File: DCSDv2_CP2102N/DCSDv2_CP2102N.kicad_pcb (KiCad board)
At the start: 2 copper layers, 37 x 27 mm, 18 parts, among them P1 USB_C_Plug_USB2.0, U1 CP2102N-Axx-xQFN28

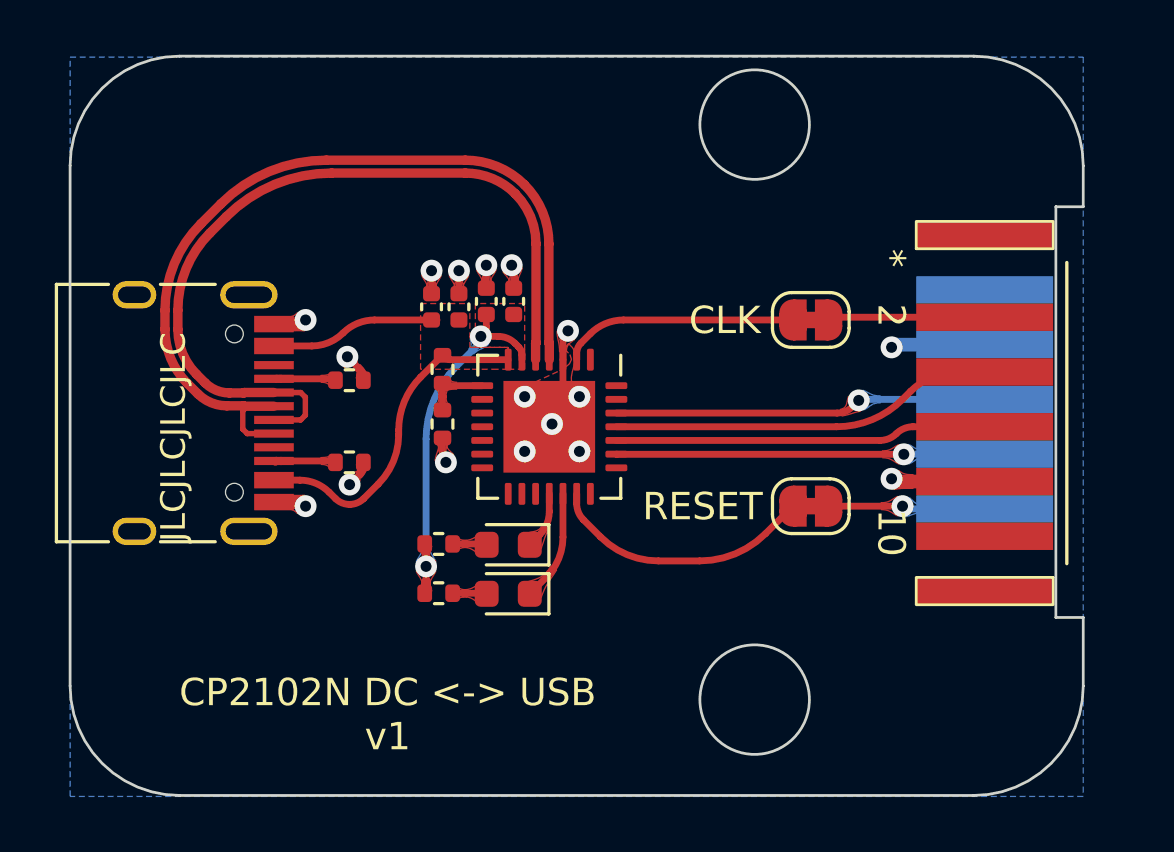
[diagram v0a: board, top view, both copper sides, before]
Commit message: Version 1.1
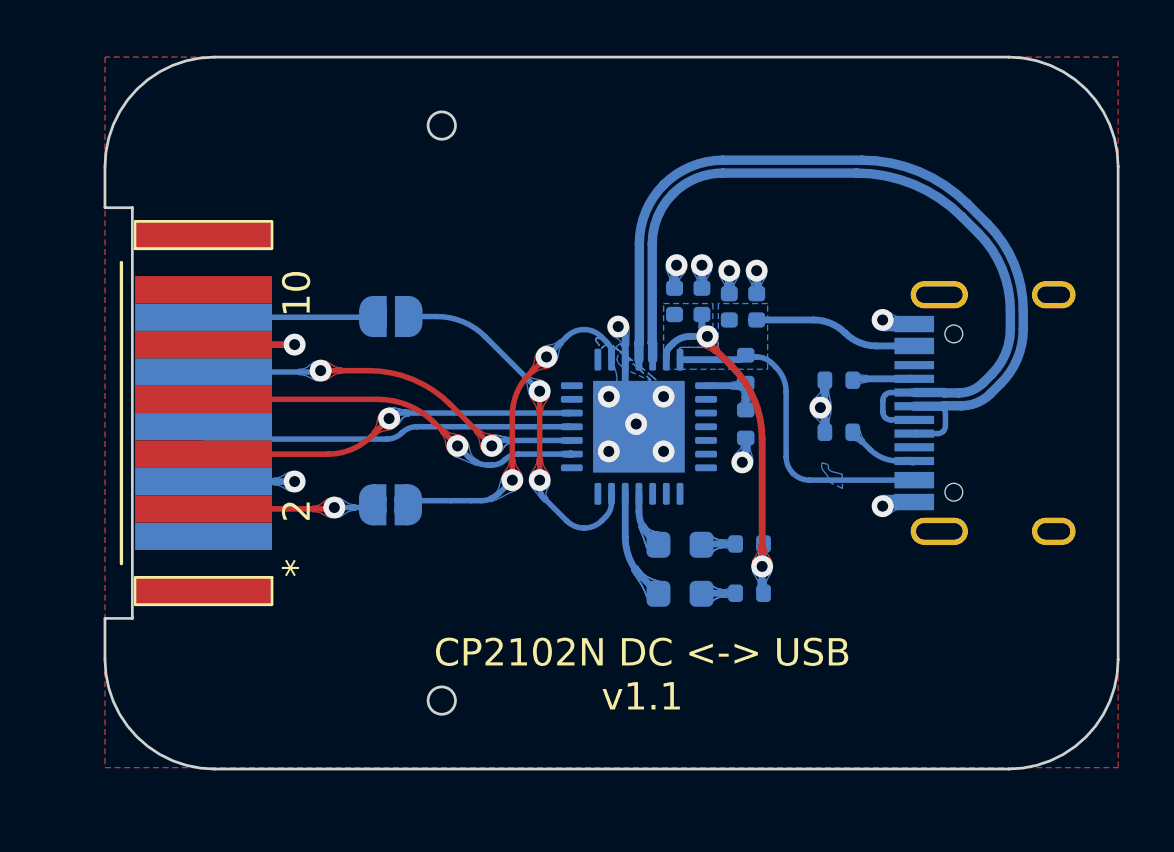
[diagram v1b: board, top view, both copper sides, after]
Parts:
- C1, C2, C3, C4, D1, D2, H1, P1, R1, R2, R3, R4, R5, R6, U1: moved to B.Cu
- JP1, JP2: footprint Jumper:SolderJumper-2_P1.3mm_Bridged_RoundedPad1.0x1.5mm -> Jumper:SolderJumper-2_P1.3mm_Open_RoundedPad1.0x1.5mm; moved to B.Cu
- moved P1 31.5 mm to (165.5, 91.8)
- moved U2 28.5 mm to (135.5, 91.8), turned to 90 degrees
- moved R2 17.9 mm to (158.7, 92.5), turned to 180 degrees
- moved R1 17.9 mm to (158.7, 90.6), turned to 180 degrees
- moved JP2 16.8 mm to (142.3, 88.3), turned to 180 degrees
- moved JP1 16.8 mm to (142.3, 95.2), turned to 180 degrees
- moved C2 11.9 mm to (155.7, 87.9)
- moved R5 11.4 mm to (155.4, 98.4), turned to 0 degrees
- moved R6 11.4 mm to (155.4, 96.6), turned to 0 degrees
- moved R3 11.1 mm to (155.3, 90.2)
- moved R4 11.1 mm to (155.3, 92.2)
- moved C1 9.87 mm to (154.7, 87.9)
- moved C3 7.87 mm to (153.7, 87.7)
- moved D1 6.27 mm to (152.9, 98.4), turned to 0 degrees
- moved D2 6.27 mm to (152.9, 96.6), turned to 0 degrees
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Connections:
- U2 pad 4: /DC_RX -> /DC_TX
- U2 pad 5: /DC_TX -> /DC_RX
- U2 pad 6: /DC_RTS -> /DC_CTS
- U2 pad 7: /DC_CTS -> /DC_RTS
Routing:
- net /CP2102N_SCK: track 8.65 -> 12.4 mm, vias 0 -> 2
- net /CP2102N_RESET: track 9.80 -> 13.4 mm, vias 0 -> 2
- net /DC_CTS: track 13.5 -> 14.4 mm
- net /DC_RTS: track 13.6 -> 14.5 mm, vias 0 -> 2
- net /DC_TX: track 13.6 -> 14.2 mm
- net /DC_SCK: track 5.73 -> 6.23 mm, vias 0 -> 1
- net /DC_RESET: track 5.73 -> 6.20 mm, vias 1 -> 0
- net GND: vias 17 -> 16
- added copper zone on B.Cu, net +3.3V
- added copper zone on B.Cu, net +5V
- added copper zone on F.Cu, net GND
- removed copper zone on F.Cu, net +3.3V
- removed copper zone on F.Cu, net +5V
- removed copper zone on B.Cu, net GND
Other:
- board size 37 x 27 mm -> 37 x 26 mm
- board text added: "CP2102N DC <-> USB v1.1"
- board text removed: "CP2102N DC <-> USB v1"
